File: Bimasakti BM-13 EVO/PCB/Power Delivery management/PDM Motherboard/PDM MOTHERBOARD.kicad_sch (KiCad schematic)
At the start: 41 parts

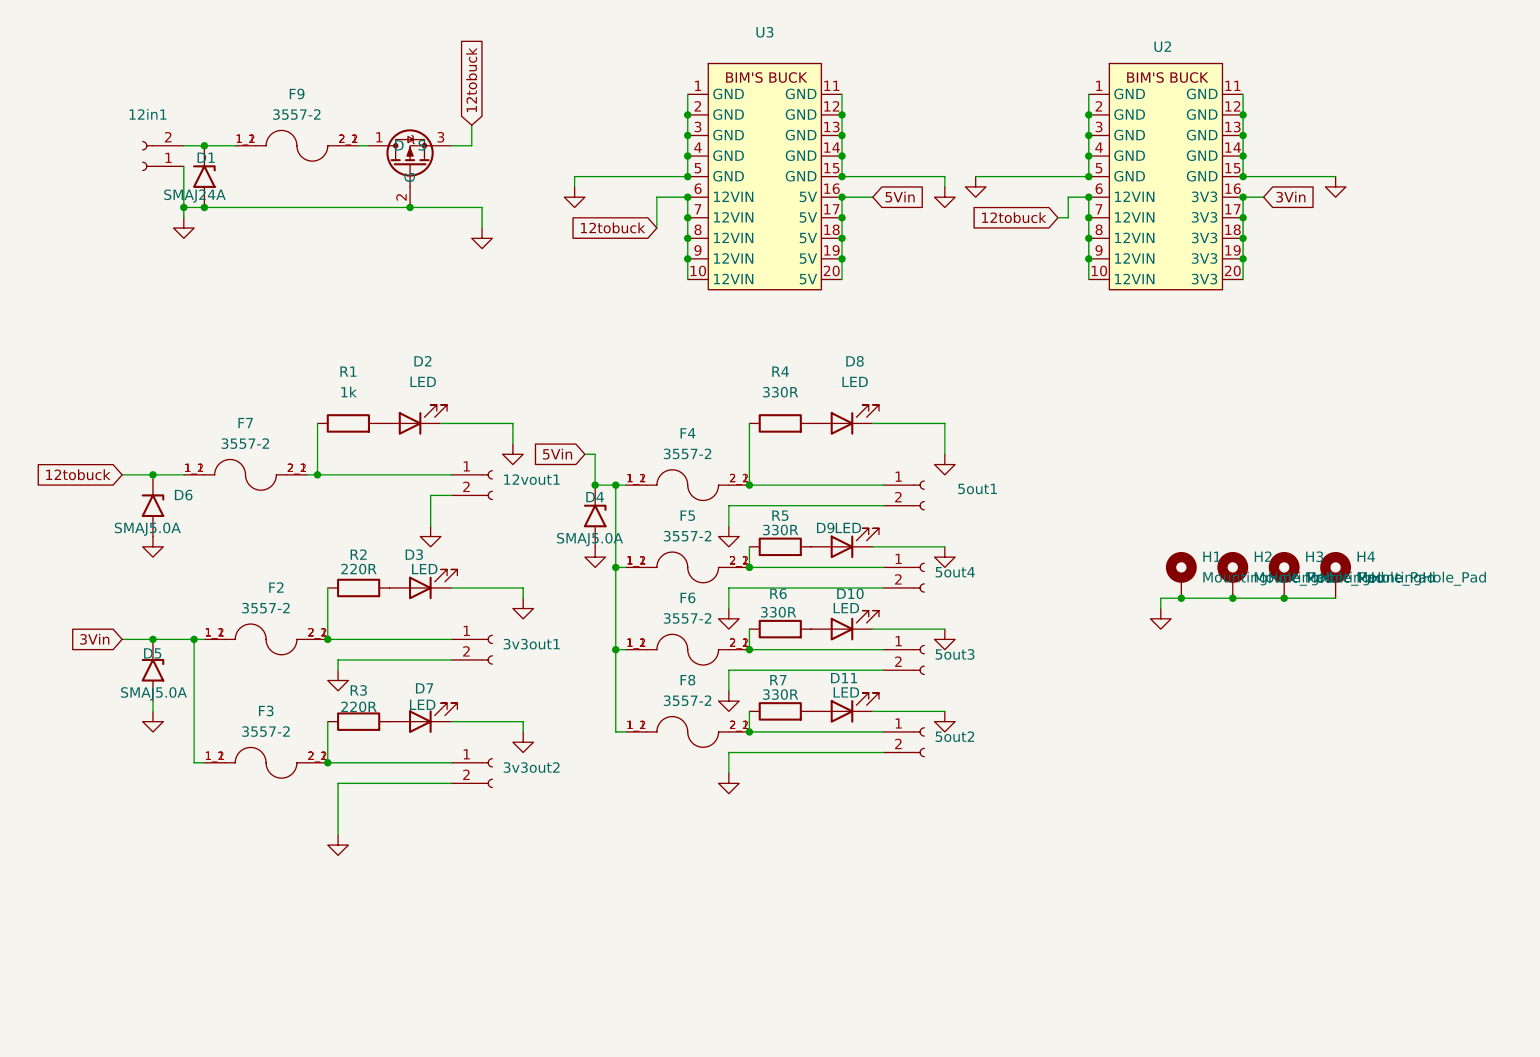
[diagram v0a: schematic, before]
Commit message: update
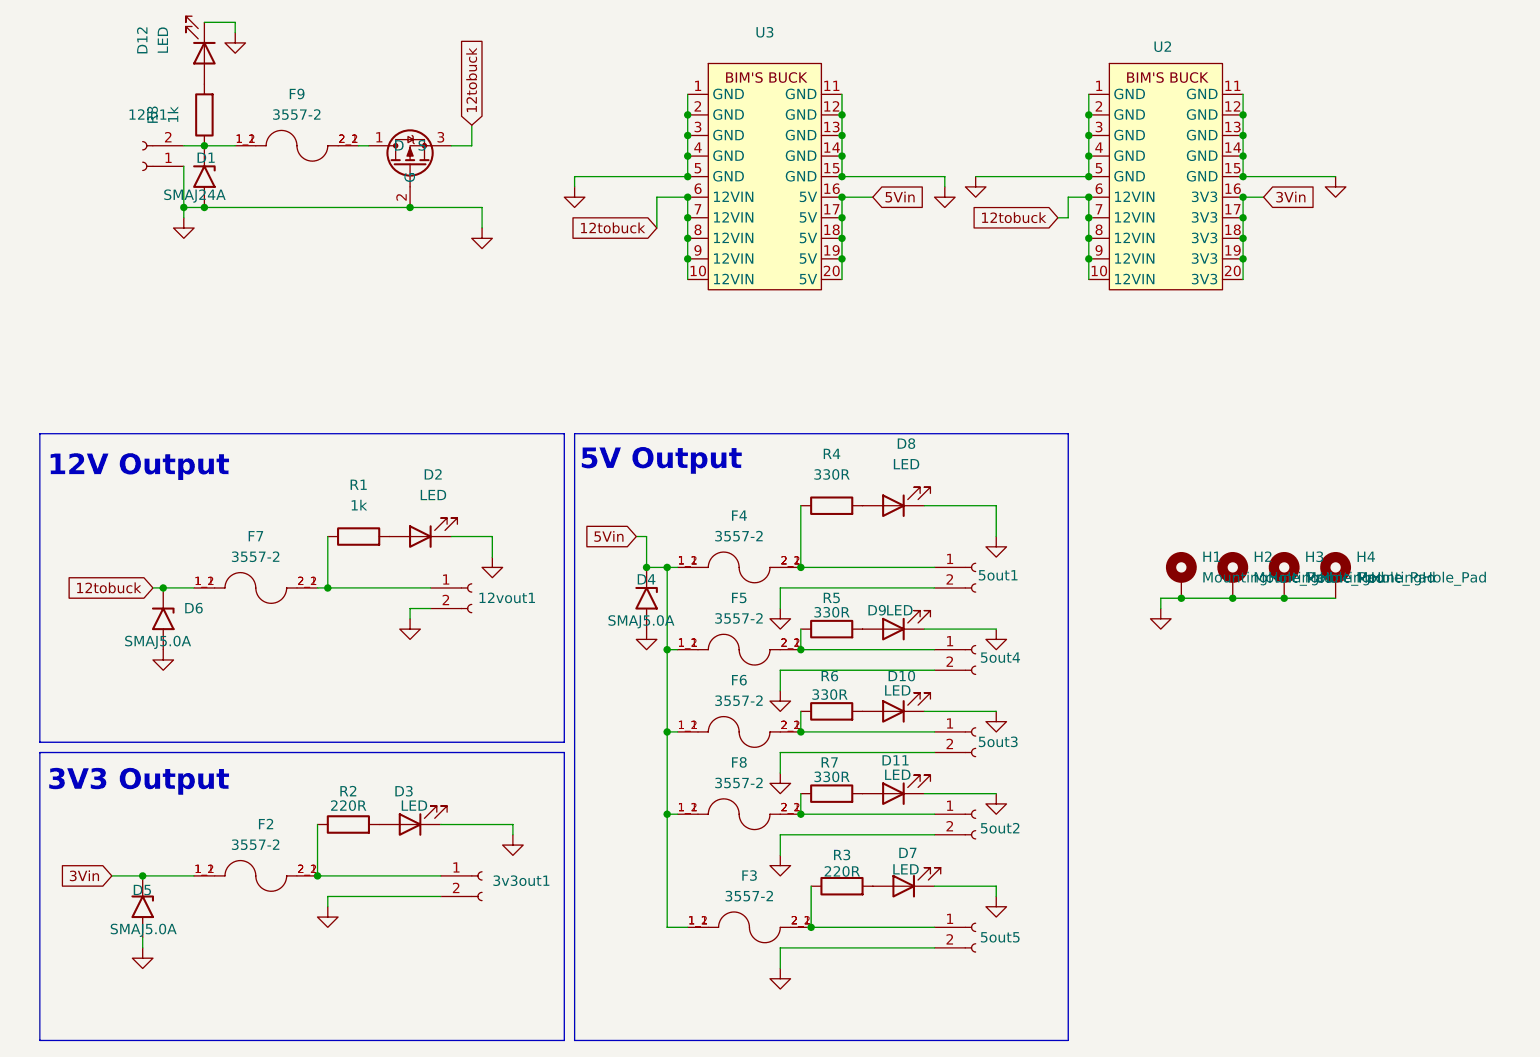
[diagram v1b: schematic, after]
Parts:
- added D12: LED, LED_SMD:LED_0805_2012Metric_Pad1.15x1.40mm_HandSolder, symbol Device:LED
- added R8: 1k, Resistor_SMD:R_0805_2012Metric_Pad1.20x1.40mm_HandSolder, symbol Device:R
- renumbered 3v3out2 to 5out5
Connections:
- net 3Vin: no longer F3.1_1, F3.1_2
- net 5Vin: now also F3.1_1, F3.1_2
- net GND: now also D12.1 (K)
- net at 12in1.2 (Pin_2), D1.1 (A1), F9.1_1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: now also R8.1
- new net: D12.2 (A), R8.2
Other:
- note added: "12V Output"
- note added: "3V3 Output"
- note added: "5V Output"
- moved on the sheet: 12vout1, 3v3out1, 5out1, 5out2, 5out3, 5out4, 5out5, D10, D11, D2, D3, D4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
